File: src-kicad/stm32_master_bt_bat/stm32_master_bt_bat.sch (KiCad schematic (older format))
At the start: 31 parts, among them J1 Conn_01x02_Male, J2 Conn_01x02_Male, J3 Conn_02x04_Odd_Even, J4 Conn_01x06_Female, Q1 Si2371EDS, SW1 SW_Push, SW2 SW_DIP_x01, U1 STM32F031F6Px, Y1 8M

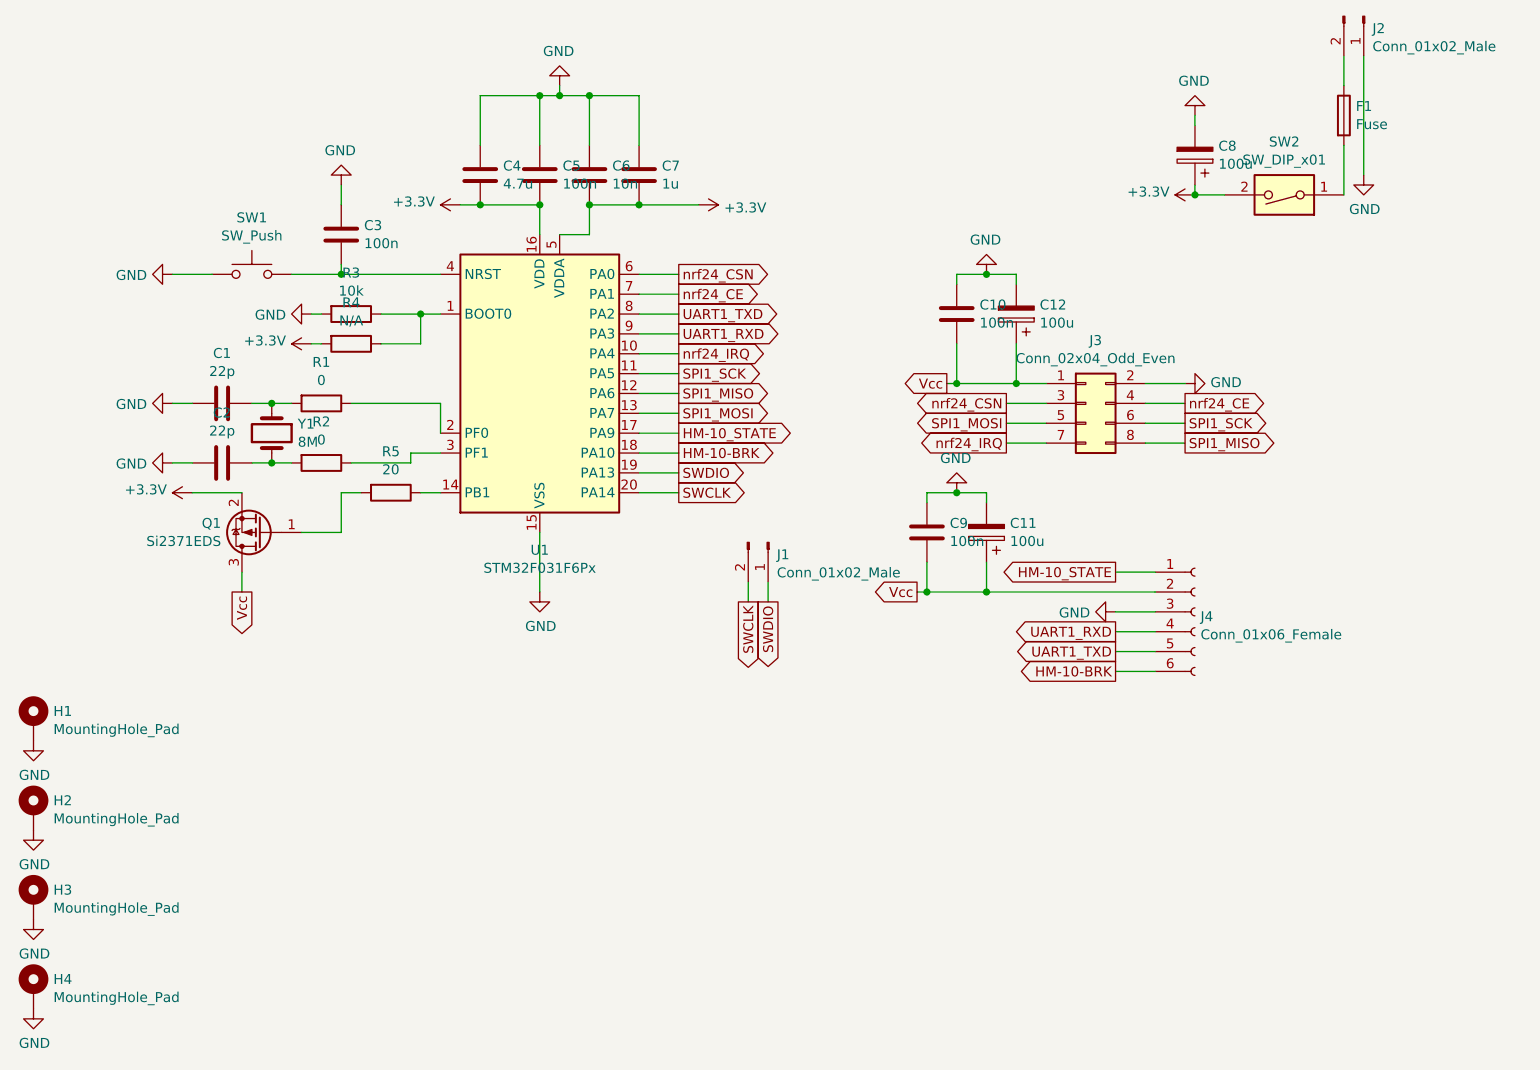
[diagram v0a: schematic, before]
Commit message: update src-kicad directory (all files)
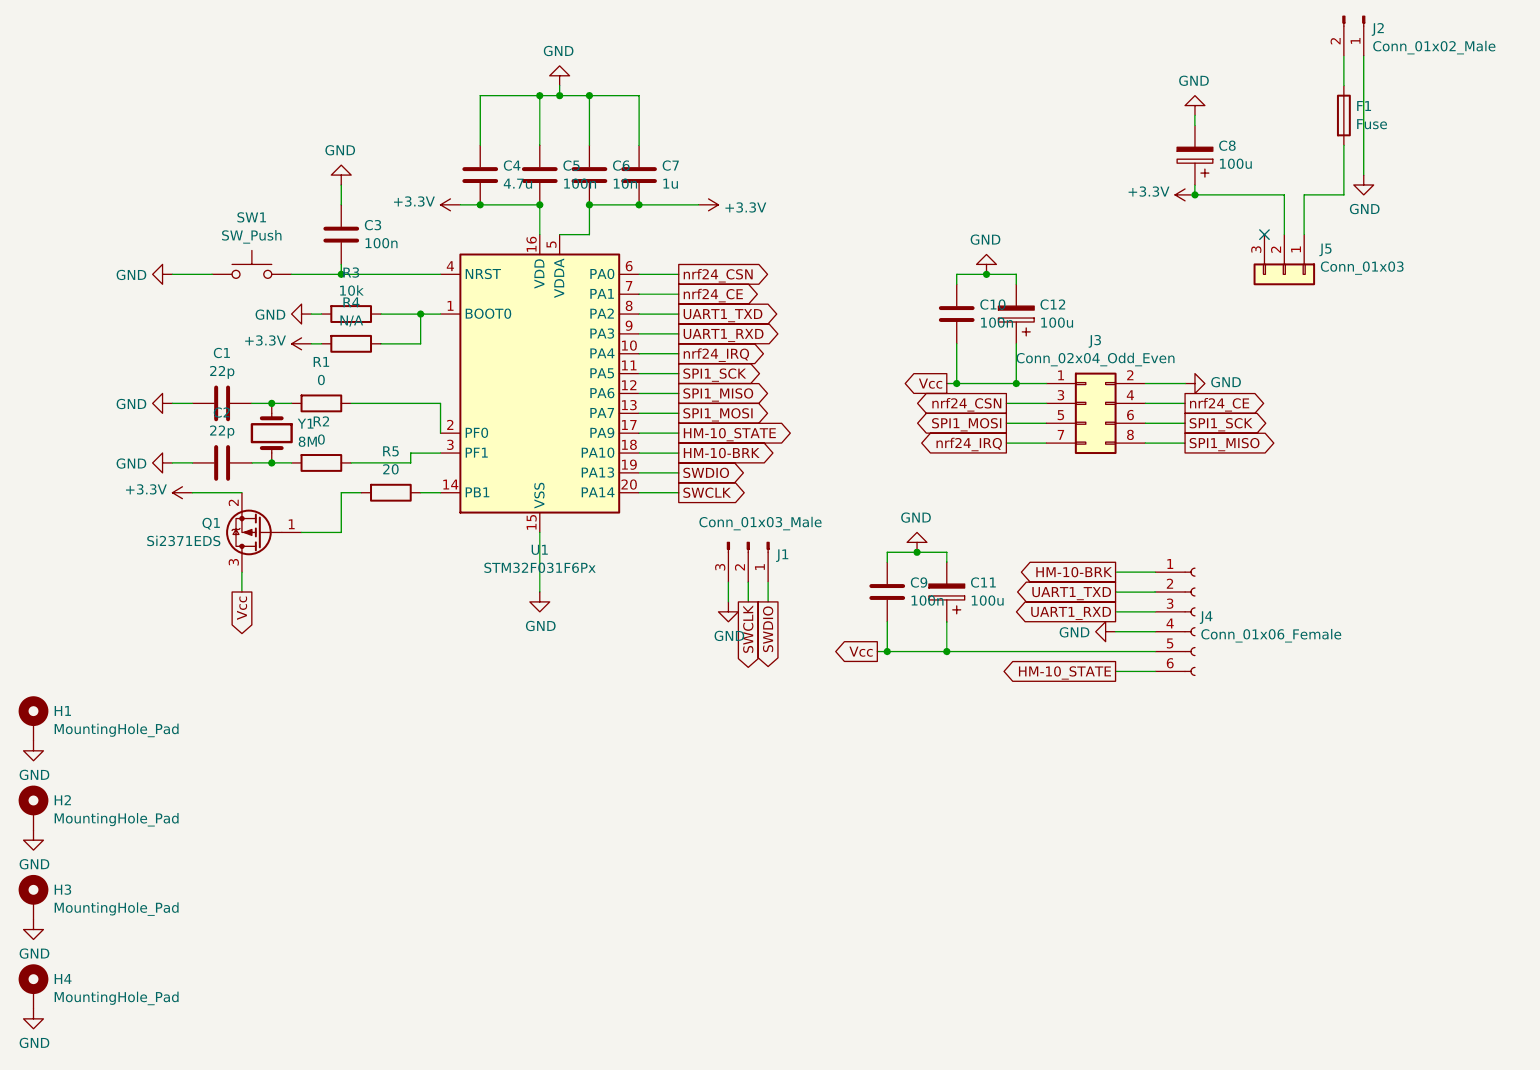
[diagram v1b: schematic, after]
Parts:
- removed J1: Conn_01x02_Male, Connector_PinHeader_2.54mm:PinHeader_1x02_P2.54mm_Vertical, symbol Connector:Conn_01x02_Male
- removed SW2: SW_DIP_x01, Button_Switch_SMD:SW_DIP_SPSTx01_Slide_6.7x4.1mm_W8.61mm_P2.54mm_LowProfile, symbol Switch:SW_DIP_x01
- added J1: Conn_01x03_Male, Connector_PinHeader_2.54mm:PinHeader_1x03_P2.54mm_Vertical, symbol Connector:Conn_01x03_Male
- added J5: Conn_01x03, przelbl1x3:PRZELBL1X3, symbol Connector_Generic:Conn_01x03
- J4: footprint Connector_PinSocket_2.54mm:PinSocket_1x06_P2.54mm_Horizontal -> Connector_PinSocket_2.54mm:PinSocket_1x06_P2.54mm_Vertical
- Y1: footprint Crystal:Crystal_SMD_HC49-SD_HandSoldering -> Crystal:Crystal_SMD_HC49-SD
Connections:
- net +3V3: now also J5.2 (Pin_2)
- net GND: now also J4.4 (Pin_4), J1.3 (Pin_3); no longer J4.3 (Pin_3)
- net HM-10-BRK: now also J4.1 (Pin_1); no longer J4.6 (Pin_6)
- net HM-10_STATE: now also J4.6 (Pin_6); no longer J4.1 (Pin_1)
- net SWCLK: now also J1.2 (Pin_2)
- net SWDIO: now also J1.1 (Pin_1)
- net UART1_RXD: now also J4.3 (Pin_3); no longer J4.4 (Pin_4)
- net UART1_TXD: now also J4.2 (Pin_2); no longer J4.5 (Pin_5)
- net Vcc: now also J4.5 (Pin_5); no longer J4.2 (Pin_2)
- net at F1.2: now also J5.1 (Pin_1)
- no-connect marks 0 -> 1
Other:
- moved on the sheet: C11, C9
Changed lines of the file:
@@
 F 0 "J4" H 7928 4976 50  0000 L CNN
 F 1 "Conn_01x06_Female" H 7928 4885 50  0000 L CNN
-F 2 "Connector_PinSocket_2.54mm:PinSocket_1x06_P2.54mm_Horizontal" H 7900 5000 50  0001 C CNN
+F 2 "Connector_PinSocket_2.54mm:PinSocket_1x06_P2.54mm_Vertical" H 7900 5000 50  0001 C CNN
 F 3 "~" H 7900 5000 50  0001 C CNN
 	1    7900 5000
 	1    0    0    -1
 $EndComp
-Text GLabel 7500 4800 0    50   Output ~ 0
+Text GLabel 7500 5300 0    50   Output ~ 0
 HM-10_STATE
 $Comp
 L power:GND #PWR017
 U 1 1 5FE8109A
-P 7500 5000
-F 0 "#PWR017" H 7500 4750 50  0001 C CNN
-F 1 "GND" V 7505 4872 50  0000 R CNN
-F 2 "" H 7500 5000 50  0001 C CNN
-F 3 "" H 7500 5000 50  0001 C CNN
-	1    7500 5000
-	0    1    1    0
-$EndComp
-Text GLabel 7500 5100 0    50   Output ~ 0
+P 7500 5100
+F 0 "#PWR017" H 7500 4850 50  0001 C CNN
+F 1 "GND" V 7505 4972 50  0000 R CNN
+F 2 "" H 7500 5100 50  0001 C CNN
+F 3 "" H 7500 5100 50  0001 C CNN
+	1    7500 5100
+	0    1    1    0
+$EndComp
+Text GLabel 7500 5000 0    50   Output ~ 0
 UART1_RXD
-Text GLabel 7500 5300 0    50   Output ~ 0
+Text GLabel 7500 4800 0    50   Output ~ 0
 HM-10-BRK
 Wire Wire Line
@@
 Wire Wire Line
 	7500 5100 7700 5100
-Wire Wire Line
-	7700 5200 7500 5200
 Wire Wire Line
 	7500 5300 7700 5300
@@
 L Device:CP C11
 U 1 1 5FE896C9
-P 6850 4600
-F 0 "C11" H 6732 4554 50  0000 R CNN
-F 1 "100u" H 6732 4645 50  0000 R CNN
-F 2 "Capacitor_SMD:CP_Elec_6.3x5.8" H 6888 4450 50  0001 C CNN
-F 3 "~" H 6850 4600 50  0001 C CNN
-	1    6850 4600
+P 6650 4900
+F 0 "C11" H 6532 4854 50  0000 R CNN
+F 1 "100u" H 6532 4945 50  0000 R CNN
+F 2 "Capacitor_SMD:CP_Elec_6.3x5.8" H 6688 4750 50  0001 C CNN
+F 3 "~" H 6650 4900 50  0001 C CNN
+	1    6650 4900
 	-1   0    0    1
 $EndComp
@@
 L Device:C C9
 U 1 1 5FE89CE9
-P 6550 4600
-F 0 "C9" H 6665 4646 50  0000 L CNN
-F 1 "100n" H 6665 4555 50  0000 L CNN
-F 2 "Capacitor_SMD:C_0805_2012Metric_Pad1.18x1.45mm_HandSolder" H 6588 4450 50  0001 C CNN
-F 3 "~" H 6550 4600 50  0001 C CNN
-	1    6550 4600
-	1    0    0    -1
-$EndComp
-Wire Wire Line
-	6500 4900 6550 4900
-Wire Wire Line
-	6550 4750 6550 4900
-Connection ~ 6550 4900
-Wire Wire Line
-	6550 4900 6850 4900
-Wire Wire Line
-	6850 4750 6850 4900
-Connection ~ 6850 4900
-Wire Wire Line
-	6850 4900 7700 4900
+P 6350 4900
+F 0 "C9" H 6465 4946 50  0000 L CNN
+F 1 "100n" H 6465 4855 50  0000 L CNN
+F 2 "Capacitor_SMD:C_0805_2012Metric_Pad1.18x1.45mm_HandSolder" H 6388 4750 50  0001 C CNN
+F 3 "~" H 6350 4900 50  0001 C CNN
+	1    6350 4900
+	1    0    0    -1
+$EndComp
+Wire Wire Line
+	6300 5200 6350 5200
+Wire Wire Line
+	6350 5050 6350 5200
+Connection ~ 6350 5200
+Wire Wire Line
+	6350 5200 6650 5200
+Wire Wire Line
+	6650 5050 6650 5200
+Connection ~ 6650 5200
 $Comp
 L power:GND #PWR014
 U 1 1 5FE8E82B
-P 6700 4400
-F 0 "#PWR014" H 6700 4150 50  0001 C CNN
-F 1 "GND" H 6705 4227 50  0000 C CNN
-F 2 "" H 6700 4400 50  0001 C CNN
-F 3 "" H 6700 4400 50  0001 C CNN
-	1    6700 4400
+P 6500 4700
+F 0 "#PWR014" H 6500 4450 50  0001 C CNN
+F 1 "GND" H 6505 4527 50  0000 C CNN
+F 2 "" H 6500 4700 50  0001 C CNN
+F 3 "" H 6500 4700 50  0001 C CNN
+	1    6500 4700
 	-1   0    0    1
 $EndComp
@@
 Connection ~ 6850 3300
 Wire Wire Line
-	6850 4450 6850 4400
-Wire Wire Line
-	6850 4400 6700 4400
-Wire Wire Line
-	6700 4400 6550 4400
-Wire Wire Line
-	6550 4400 6550 4450
-Connection ~ 6700 4400
+	6650 4750 6650 4700
+Wire Wire Line
+	6650 4700 6500 4700
+Wire Wire Line
+	6500 4700 6350 4700
+Wire Wire Line
+	6350 4700 6350 4750
+Connection ~ 6500 4700
 $Comp
 L Connector:Conn_01x02_Male J2
@@
 Wire Wire Line
 	5100 4000 5300 4000
-Text GLabel 7500 5200 0    50   Output ~ 0
+Text GLabel 7500 4900 0    50   Output ~ 0
 UART1_TXD
 Text GLabel 5300 3500 2    50   Output ~ 0
@@
 F 0 "Y1" V 3204 4231 50  0000 L CNN
 F 1 "8M" V 3295 4231 50  0000 L CNN
-F 2 "Crystal:Crystal_SMD_HC49-SD_HandSoldering" H 3250 4100 50  0001 C CNN
+F 2 "Crystal:Crystal_SMD_HC49-SD" H 3250 4100 50  0001 C CNN
 F 3 "~" H 3250 4100 50  0001 C CNN
 	1    3250 4100
@@
 Wire Wire Line
 	5300 4400 5100 4400
-$Comp
-L Connector:Conn_01x02_Male J1
-U 1 1 5FF2A3AF
-P 5750 4650
-F 0 "J1" V 5812 4694 50  0000 L CNN
-F 1 "Conn_01x02_Male" V 5903 4694 50  0000 L CNN
-F 2 "Connector_PinHeader_2.54mm:PinHeader_1x02_P2.54mm_Vertical" H 5750 4650 50  0001 C CNN
-F 3 "~" H 5750 4650 50  0001 C CNN
-	1    5750 4650
-	0    1    1    0
-$EndComp
 Text GLabel 5750 4950 3    50   Output ~ 0
 SWDIO
@@
 Wire Wire Line
 	5650 4950 5650 4850
-$Comp
-L Switch:SW_DIP_x01 SW2
-U 1 1 5FF6014A
-P 8350 2900
-F 0 "SW2" H 8350 2633 50  0000 C CNN
-F 1 "SW_DIP_x01" H 8350 2724 50  0000 C CNN
-F 2 "Button_Switch_SMD:SW_DIP_SPSTx01_Slide_6.7x4.1mm_W8.61mm_P2.54mm_LowProfile" H 8350 2900 50  0001 C CNN
-F 3 "~" H 8350 2900 50  0001 C CNN
-	1    8350 2900
-	-1   0    0    1
-$EndComp
 Wire Wire Line
 	8650 2650 8650 2900
-Wire Wire Line
-	8050 2900 7900 2900
 $Comp
 L Device:CP C8
@@
 Wire Wire Line
 	3100 4400 2850 4400
-Wire Wire Line
-	3100 4800 3100 4900
 Text GLabel 3100 4900 3    50   Output ~ 0
 Vcc
-Text GLabel 6500 4900 0    50   Output ~ 0
+Text GLabel 6300 5200 0    50   Output ~ 0
 Vcc
 Text GLabel 6650 3850 0    50   Output ~ 0
@@
 	1    0    0    -1
 $EndComp
+$Comp
+L Connector_Generic:Conn_01x03 J5
+U 1 1 5FF7B66B
+P 8350 3300
+F 0 "J5" V 8222 3480 50  0000 L CNN
+F 1 "Conn_01x03" V 8313 3480 50  0000 L CNN
+F 2 "przelbl1x3:PRZELBL1X3" H 8350 3300 50  0001 C CNN
+F 3 "~" H 8350 3300 50  0001 C CNN
+	1    8350 3300
+	0    1    1    0
+$EndComp
+Wire Wire Line
+	8650 2900 8450 2900
+Wire Wire Line
+	8450 2900 8450 3100
+Wire Wire Line
+	8350 3100 8350 2900
+Wire Wire Line
+	7900 2900 8350 2900
+NoConn ~ 8250 3100
+$Comp
+L Connector:Conn_01x03_Male J1
+U 1 1 5FFCE0E1
+P 5650 4650
+F 0 "J1" V 5712 4794 50  0000 L CNN
+F 1 "Conn_01x03_Male" V 5550 4400 50  0000 L CNN
+F 2 "Connector_PinHeader_2.54mm:PinHeader_1x03_P2.54mm_Vertical" H 5650 4650 50  0001 C CNN
+F 3 "~" H 5650 4650 50  0001 C CNN
+	1    5650 4650
+	0    1    1    0
+$EndComp
+$Comp
+L power:GND #PWR019
+U 1 1 5FFD868C
+P 5550 4950
+F 0 "#PWR019" H 5550 4700 50  0001 C CNN
+F 1 "GND" H 5555 4777 50  0000 C CNN
+F 2 "" H 5550 4950 50  0001 C CNN
+F 3 "" H 5550 4950 50  0001 C CNN
+	1    5550 4950
+	1    0    0    -1
+$EndComp
+Wire Wire Line
+	5550 4950 5550 4850
+Wire Wire Line
+	3100 4800 3100 4900
+Wire Wire Line
+	7700 4900 7500 4900
+Wire Wire Line
+	6650 5200 7700 5200
 $EndSCHEMATC
